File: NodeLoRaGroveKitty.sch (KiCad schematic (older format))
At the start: 38 parts, among them P1 PICKIT PROGRAMMER, P2 Battery, P3 A0, P4 D9, P5 USB-Serial, P6 I2C, SW1 SW_BOOT, SW2 SW_RESET, U1 AP2114, U2 MCP73831T-2ATI/OT, U3 ESP-12E

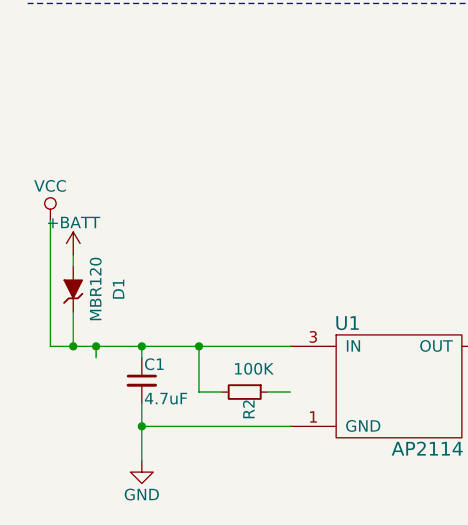
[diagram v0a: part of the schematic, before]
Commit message: Add mbr120
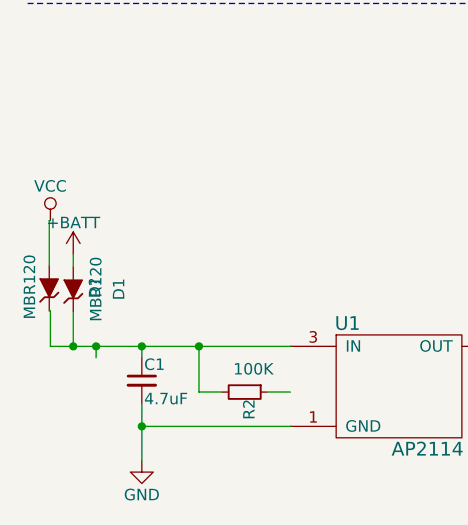
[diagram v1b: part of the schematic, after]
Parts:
- added D?: MBR120, Diodes_SMD:SOD-123, symbol ZENERsmall
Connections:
- net VCC: now also D?.2 (A); no longer C1.1, D1.1 (K), R2.2, U1.3 (IN)
- new net: C1.1, D1.1 (K), D?.1 (K), R2.2, U1.3 (IN)
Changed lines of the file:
@@
 	1    0    0    -1
+$EndComp
+$Comp
+L ZENERsmall D?
+U 1 1 58924335
+P 595 5845
+F 0 "D?" H 595 5645 50  0000 C CNN
+F 1 "MBR120" H 600 5930 50  0000 C CNN
+F 2 "Diodes_SMD:SOD-123" H 595 5845 50  0001 C CNN
+F 3 "" H 595 5845 50  0000 C CNN
+F 4 "NRVB120VLSFT1G" H 595 5845 60  0001 C CNN "manf#"
+	1    595  5845
+	0    -1   -1   0
 $EndComp
 Wire Wire Line
@@
 	2900 6100 2900 6000
 Connection ~ 700  6100
-Wire Wire Line
-	600  5550 600  6100
 Connection ~ 1000 6450
 Wire Wire Line
@@
 Wire Wire Line
 	2600 6100 2900 6100
+Wire Wire Line
+	595  5745 595  5550
+Wire Wire Line
+	595  5550 600  5550
+Wire Wire Line
+	600  6100 600  5945
+Wire Wire Line
+	600  5945 595  5945
 $EndSCHEMATC
